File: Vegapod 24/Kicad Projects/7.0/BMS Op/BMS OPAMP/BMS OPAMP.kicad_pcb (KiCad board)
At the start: 2 copper layers, 85.1 x 85.1 mm, 183 parts, among them J1 CHG/DSCHG CTRL, J10 Port Selector, J11 Port Selector, J12 FTDI, J18 Conn_02x06_Odd_Even, J2 CHG/DSCHG CTRL CMP (SHORT DAT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, J3 Data IN/OUT, J4 Data IN/OUT, J5 Port Selector, J6 Port Selector, J7 Port Selector, J8 Port Selector, J9 Balance Connector, Q1 MMBT3906/FDN358P, Q10 MMBT3904/AM2304/AO3400, Q2 MMBT3904/AM2304/AO3400, Q3 MMBT3904/AM2304/AO3400, Q4 MMBT3904/AM2304/AO3400, Q5 MMBT3904/AM2304/AO3400, Q6 MMBT3904/AM2304/AO3400, Q7 MMBT3904/AM2304/AO3400, Q8 MMBT3904/AM2304/AO3400, Q9 MMBT3904/AM2304/AO3400, U1 PC817, U10 LM324, U11 LM324, U12 PC817, U2 PC817, U3 PC817, U4 PC817, U6 6N137, U7 6N137, U8 LM78M05_TO252, U9 LM324

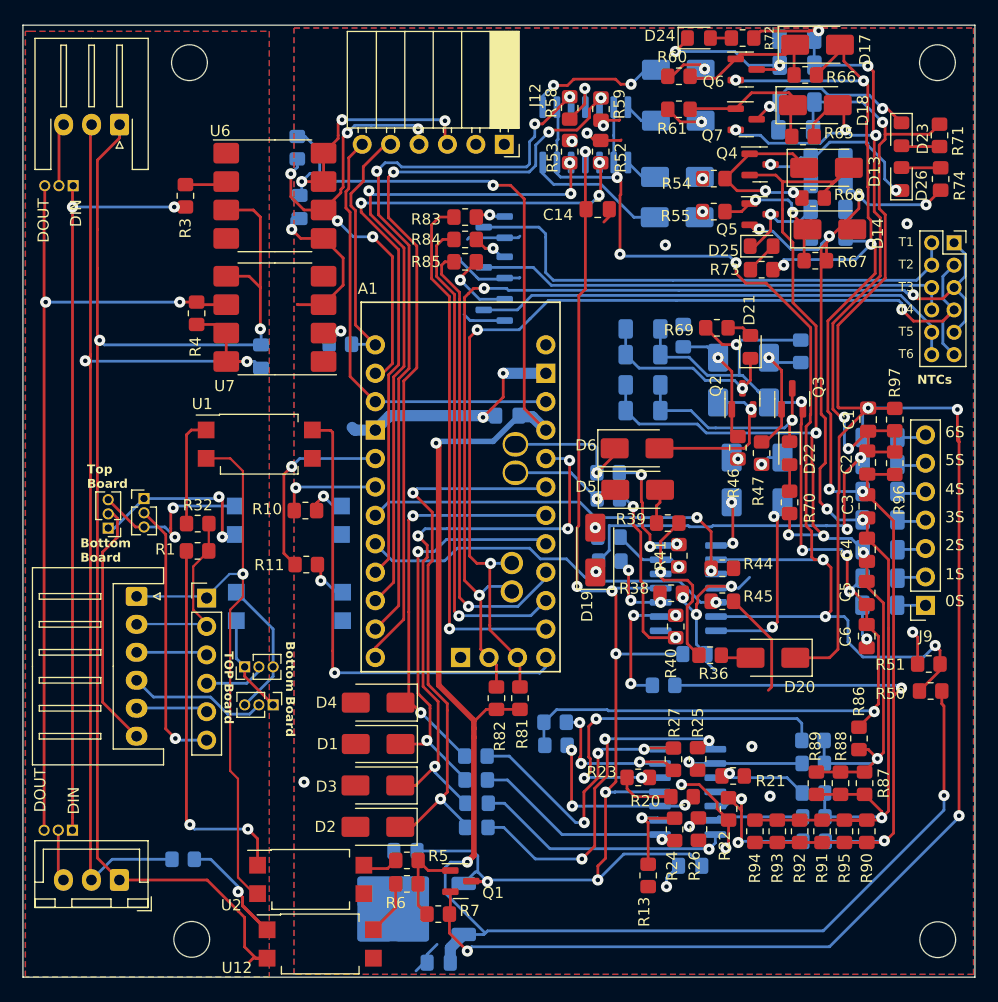
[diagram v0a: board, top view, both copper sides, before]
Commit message: BMS PCB
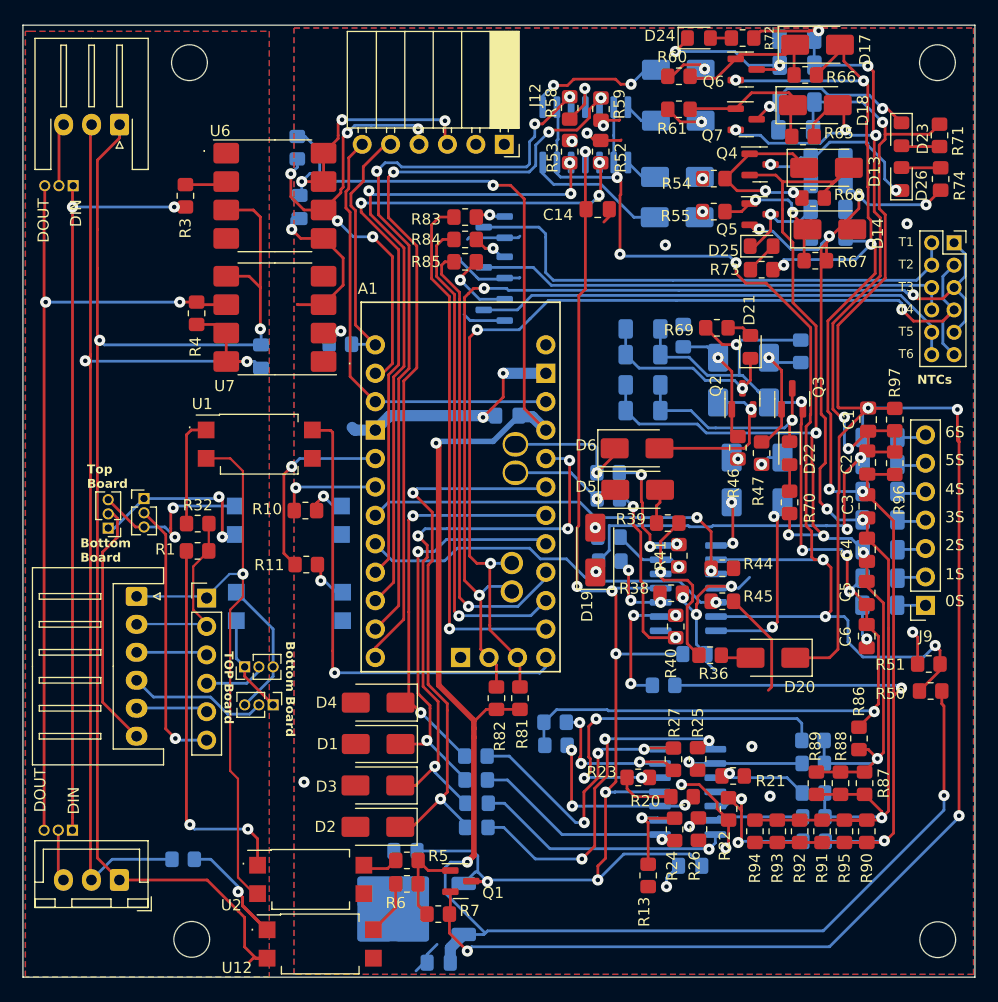
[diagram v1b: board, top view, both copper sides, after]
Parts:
- D10, D13, D14, D17, D18, D9: value 12V Z -> 5V Z
